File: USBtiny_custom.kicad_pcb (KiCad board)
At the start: 2 copper layers, 50.9 x 27.7 mm, 28 parts, among them J1 USB_B_Micro, J2 USB_A, J3 AVR-ISP-6, SW1 SW_SPDT, U1 ATtiny2313-20SU, U2 74125, Y1 12M

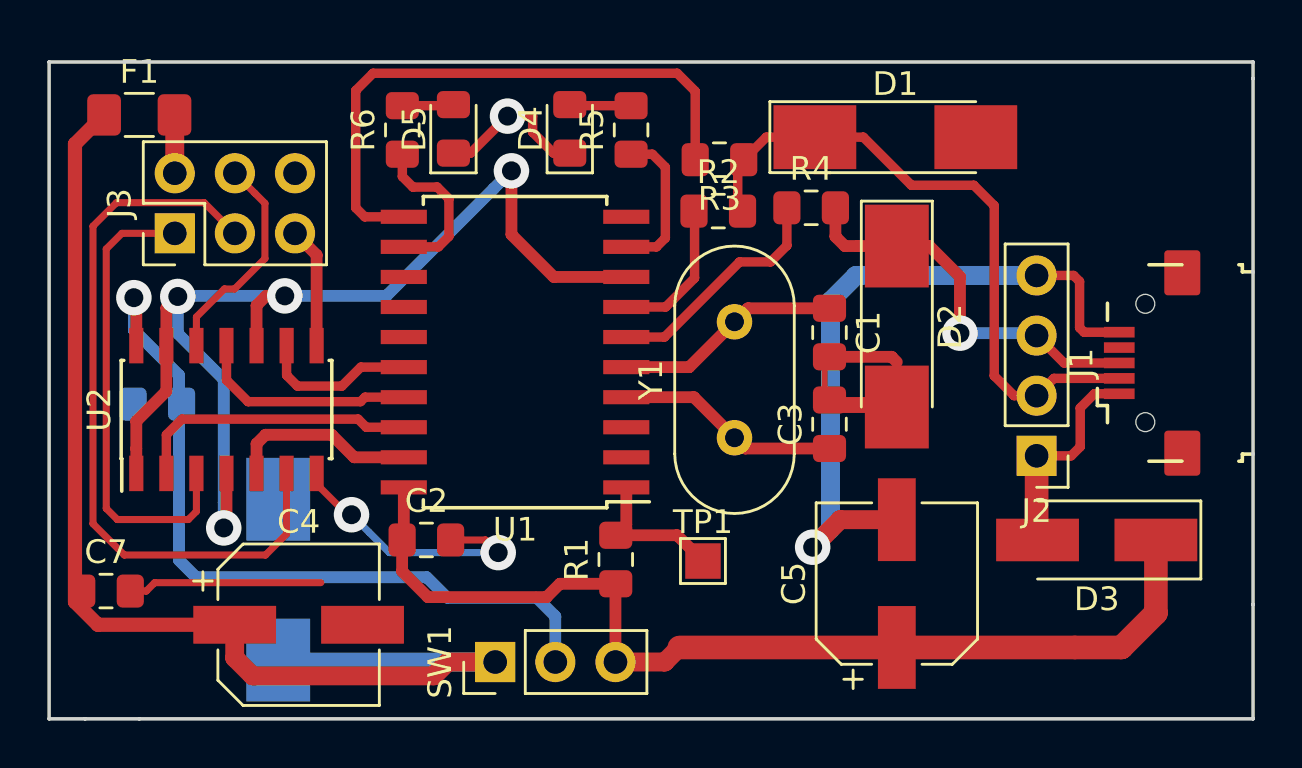
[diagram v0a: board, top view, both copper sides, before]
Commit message: kicad meta update
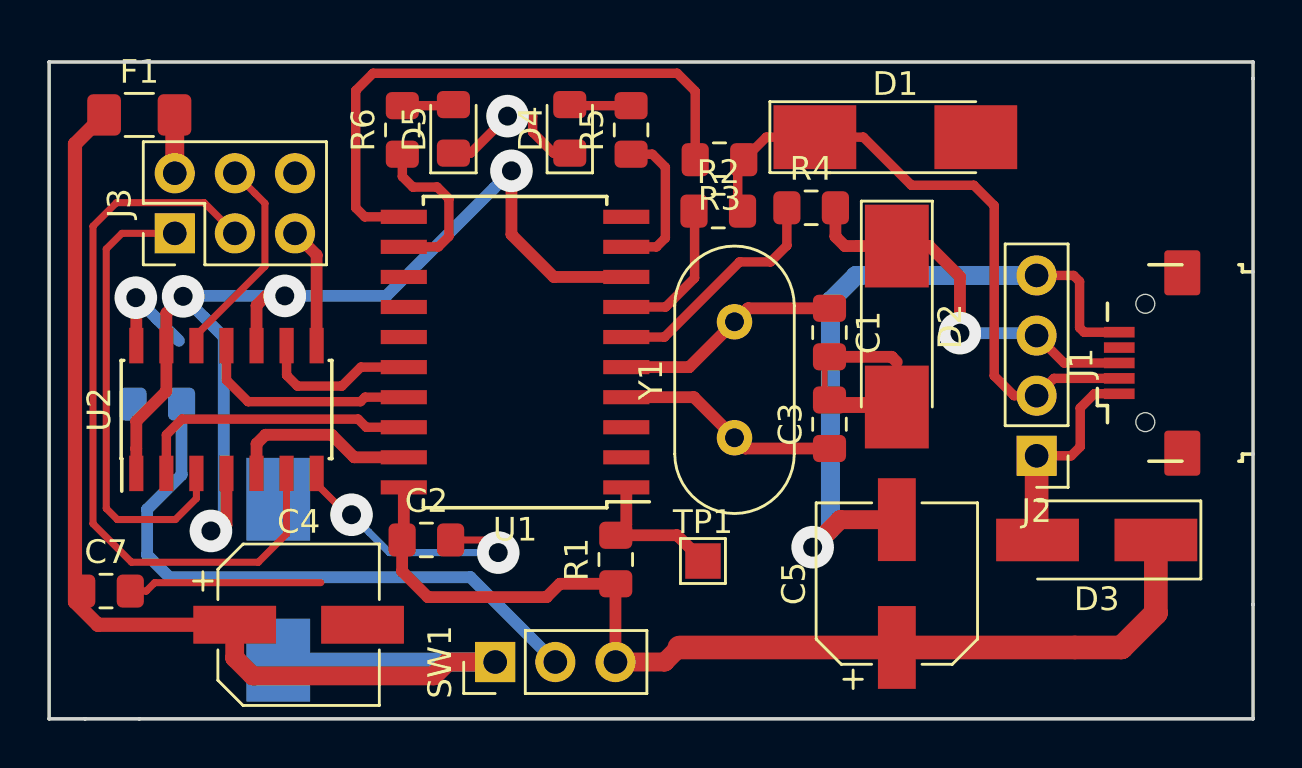
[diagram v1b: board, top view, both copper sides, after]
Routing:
- net VDD: track 32.8 -> 30.7 mm
